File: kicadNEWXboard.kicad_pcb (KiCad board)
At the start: 2 copper layers, 89.7 x 38.1 mm, 24 parts, among them SW1 SW_Push, U1 ATmega32U4-AU, Y1 16MHz

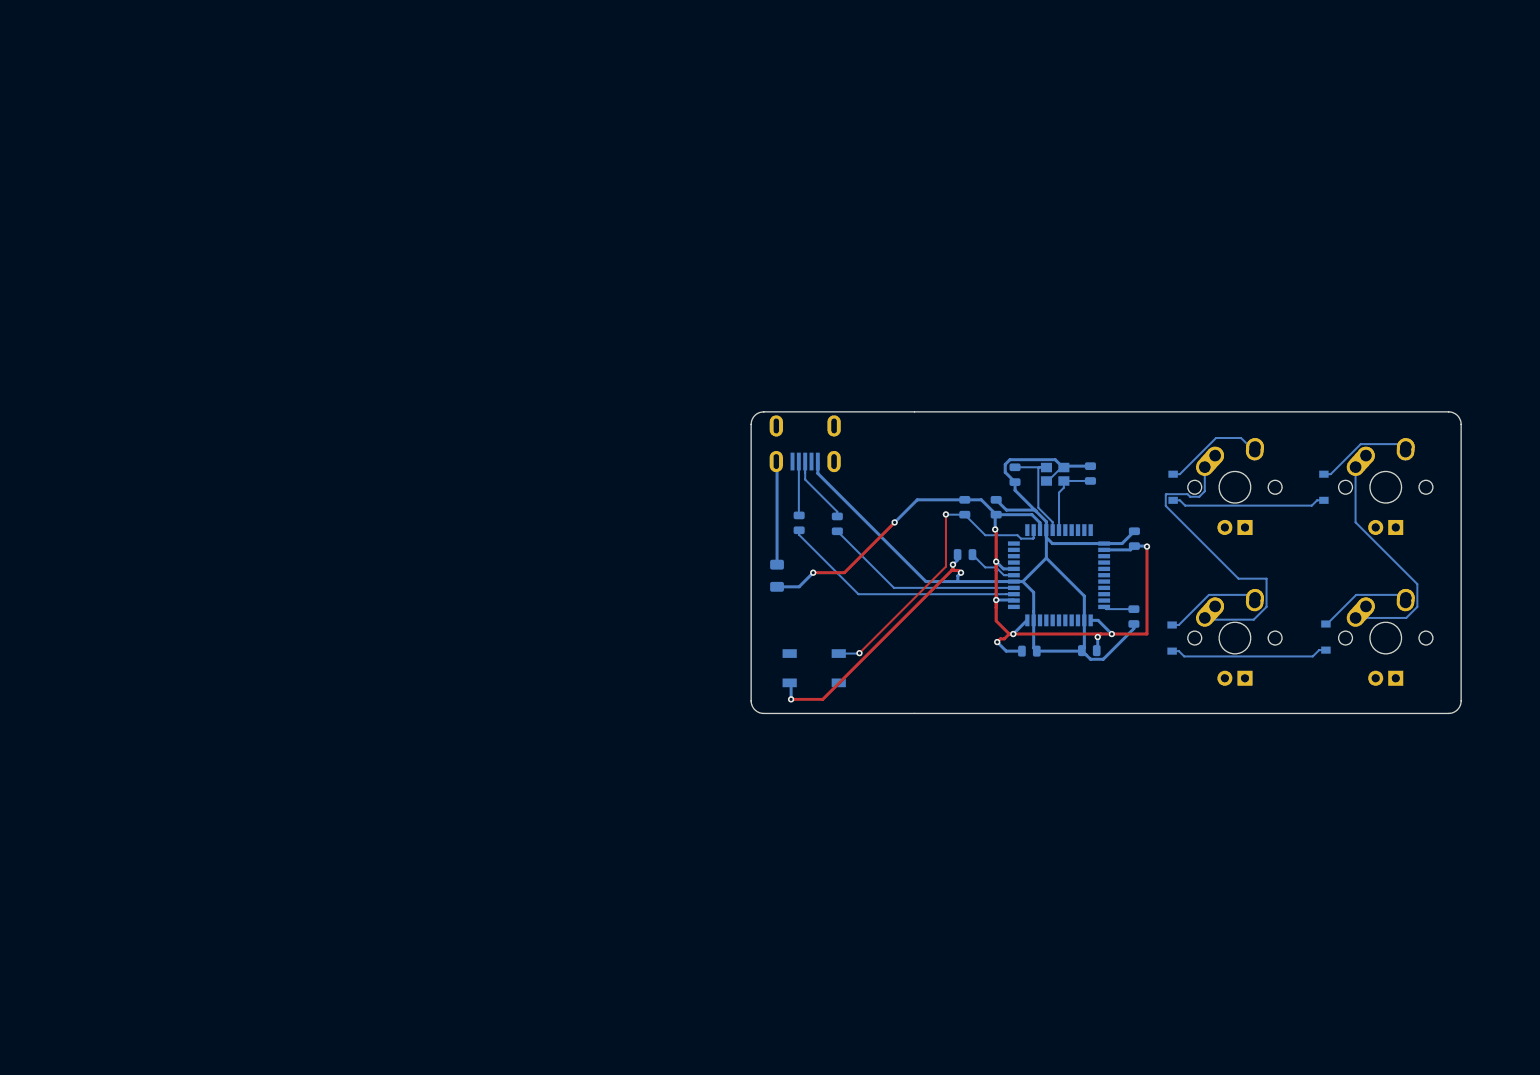
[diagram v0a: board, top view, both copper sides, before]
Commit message: SVG
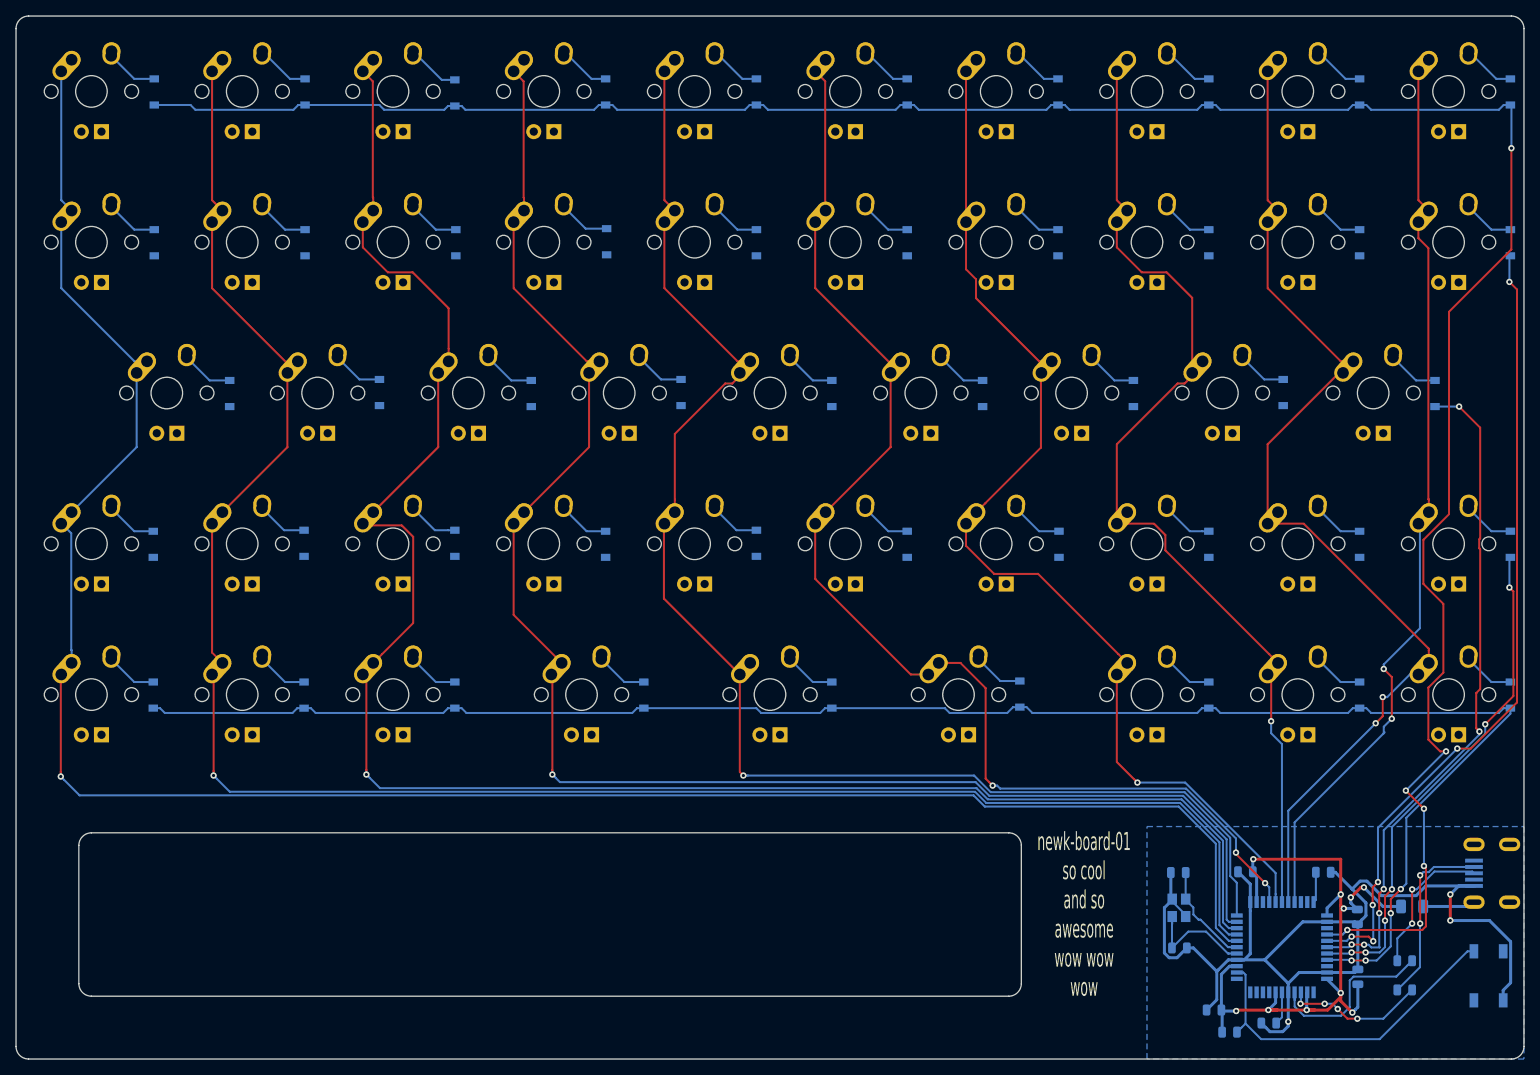
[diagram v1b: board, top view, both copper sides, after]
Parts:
- added D10: SOD-123, Diode_SMD:D_SOD-123, B.Cu at (71.3, 112.0)
- added D11: SOD-123, Diode_SMD:D_SOD-123, B.Cu at (90.4, 35.9)
- added D12: SOD-123, Diode_SMD:D_SOD-123, B.Cu at (90.5, 54.8)
- added D13: SOD-123, Diode_SMD:D_SOD-123, B.Cu at (100.0, 73.9)
- added D14: SOD-123, Diode_SMD:D_SOD-123, B.Cu at (90.4, 92.8)
- added D15: SOD-123, Diode_SMD:D_SOD-123, B.Cu at (90.4, 112.0)
- added D16: SOD-123, Diode_SMD:D_SOD-123, B.Cu at (109.4, 35.8)
- added D17: SOD-123, Diode_SMD:D_SOD-123, B.Cu at (109.5, 54.7)
- added D18: SOD-123, Diode_SMD:D_SOD-123, B.Cu at (118.9, 73.8)
- added D19: SOD-123, Diode_SMD:D_SOD-123, B.Cu at (109.4, 92.9)
- added D20: SOD-123, Diode_SMD:D_SOD-123, B.Cu at (114.2, 112.0)
- added D21: SOD-123, Diode_SMD:D_SOD-123, B.Cu at (128.5, 35.8)
- added D22: SOD-123, Diode_SMD:D_SOD-123, B.Cu at (128.5, 54.8)
- added D23: SOD-123, Diode_SMD:D_SOD-123, B.Cu at (138.0, 73.9)
- added D24: SOD-123, Diode_SMD:D_SOD-123, B.Cu at (128.5, 92.8)
- added D25: SOD-123, Diode_SMD:D_SOD-123, B.Cu at (138.0, 112.0)
- added D26: SOD-123, Diode_SMD:D_SOD-123, B.Cu at (147.5, 35.8)
- added D27: SOD-123, Diode_SMD:D_SOD-123, B.Cu at (147.5, 54.8)
- added D28: SOD-123, Diode_SMD:D_SOD-123, B.Cu at (157.0, 73.9)
- added D29: SOD-123, Diode_SMD:D_SOD-123, B.Cu at (147.5, 92.9)
- added D30: SOD-123, Diode_SMD:D_SOD-123, B.Cu at (161.7, 111.9)
- added D31: SOD-123, Diode_SMD:D_SOD-123, B.Cu at (166.6, 35.8)
- added D32: SOD-123, Diode_SMD:D_SOD-123, B.Cu at (166.6, 54.8)
- added D33: SOD-123, Diode_SMD:D_SOD-123, B.Cu at (176.1, 73.9)
- added D34: SOD-123, Diode_SMD:D_SOD-123, B.Cu at (166.7, 92.9)
- added D35: SOD-123, Diode_SMD:D_SOD-123, B.Cu at (185.6, 112.0)
- added D36: SOD-123, Diode_SMD:D_SOD-123, B.Cu at (185.6, 35.8)
- added D37: SOD-123, Diode_SMD:D_SOD-123, B.Cu at (185.6, 54.8)
- added D38: SOD-123, Diode_SMD:D_SOD-123, B.Cu at (195.0, 73.8)
- added D39: SOD-123, Diode_SMD:D_SOD-123, B.Cu at (185.6, 92.9)
- added D40: SOD-123, Diode_SMD:D_SOD-123, B.Cu at (204.7, 112.0)
- added D41: SOD-123, Diode_SMD:D_SOD-123, B.Cu at (204.7, 35.8)
- added D42: SOD-123, Diode_SMD:D_SOD-123, B.Cu at (204.7, 54.8)
- added D43: SOD-123, Diode_SMD:D_SOD-123, B.Cu at (214.2, 73.9)
- added D44: SOD-123, Diode_SMD:D_SOD-123, B.Cu at (204.7, 92.9)
- added D45: SOD-123, Diode_SMD:D_SOD-123, B.Cu at (223.7, 112.0)
- added D46: SOD-123, Diode_SMD:D_SOD-123, B.Cu at (223.7, 35.8)
- added D47: SOD-123, Diode_SMD:D_SOD-123, B.Cu at (223.7, 54.8)
- added D48: SOD-123, Diode_SMD:D_SOD-123, B.Cu at (223.7, 92.9)
- added D5: SOD-123, Diode_SMD:D_SOD-123, B.Cu at (61.9, 73.9)
- added D6: SOD-123, Diode_SMD:D_SOD-123, B.Cu at (52.3, 92.9)
- added D7: SOD-123, Diode_SMD:D_SOD-123, B.Cu at (52.3, 112.0)
- added D8: SOD-123, Diode_SMD:D_SOD-123, B.Cu at (80.8, 73.8)
- added D9: SOD-123, Diode_SMD:D_SOD-123, B.Cu at (71.3, 92.8)
- added MX10: MX-NoLED, MX_Alps_Hybrid:MX-1U, F.Cu at (63.5, 111.9)
- added MX11: MX-NoLED, MX_Alps_Hybrid:MX-1U, F.Cu at (82.5, 35.7)
- added MX12: MX-NoLED, MX_Alps_Hybrid:MX-1U, F.Cu at (82.5, 54.8)
- added MX13: MX-NoLED, MX_Alps_Hybrid:MX-1U, F.Cu at (92.1, 73.8)
- added MX14: MX-NoLED, MX_Alps_Hybrid:MX-1U, F.Cu at (82.5, 92.9)
- added MX15: MX-NoLED, MX_Alps_Hybrid:MX-1U, F.Cu at (82.5, 111.9)
- added MX16: MX-NoLED, MX_Alps_Hybrid:MX-1U, F.Cu at (101.6, 35.7)
- added MX17: MX-NoLED, MX_Alps_Hybrid:MX-1U, F.Cu at (101.6, 54.8)
- added MX18: MX-NoLED, MX_Alps_Hybrid:MX-1U, F.Cu at (111.1, 73.8)
- added MX19: MX-NoLED, MX_Alps_Hybrid:MX-1U, F.Cu at (101.6, 92.9)
- added MX20: MX-NoLED, MX_Alps_Hybrid:MX-1U, F.Cu at (106.4, 111.9)
- added MX21: MX-NoLED, MX_Alps_Hybrid:MX-1U, F.Cu at (120.7, 35.7)
- added MX22: MX-NoLED, MX_Alps_Hybrid:MX-1U, F.Cu at (120.7, 54.8)
- added MX23: MX-NoLED, MX_Alps_Hybrid:MX-1U, F.Cu at (130.2, 73.8)
- added MX24: MX-NoLED, MX_Alps_Hybrid:MX-1U, F.Cu at (120.7, 92.9)
- added MX25: MX-NoLED, MX_Alps_Hybrid:MX-1U, F.Cu at (130.2, 111.9)
- added MX26: MX-NoLED, MX_Alps_Hybrid:MX-1U, F.Cu at (139.7, 35.7)
- added MX27: MX-NoLED, MX_Alps_Hybrid:MX-1U, F.Cu at (139.7, 54.8)
- added MX28: MX-NoLED, MX_Alps_Hybrid:MX-1U, F.Cu at (149.2, 73.8)
- added MX29: MX-NoLED, MX_Alps_Hybrid:MX-1U, F.Cu at (139.7, 92.9)
- added MX30: MX-NoLED, MX_Alps_Hybrid:MX-1U, F.Cu at (154.0, 111.9)
- added MX31: MX-NoLED, MX_Alps_Hybrid:MX-1U, F.Cu at (158.8, 35.7)
- added MX32: MX-NoLED, MX_Alps_Hybrid:MX-1U, F.Cu at (158.8, 54.8)
- added MX33: MX-NoLED, MX_Alps_Hybrid:MX-1U, F.Cu at (168.3, 73.8)
- added MX34: MX-NoLED, MX_Alps_Hybrid:MX-1U, F.Cu at (158.8, 92.9)
- added MX35: MX-NoLED, MX_Alps_Hybrid:MX-1U, F.Cu at (177.8, 111.9)
- added MX36: MX-NoLED, MX_Alps_Hybrid:MX-1U, F.Cu at (177.8, 35.7)
- added MX37: MX-NoLED, MX_Alps_Hybrid:MX-1U, F.Cu at (177.8, 54.8)
- added MX38: MX-NoLED, MX_Alps_Hybrid:MX-1U, F.Cu at (187.3, 73.8)
- added MX39: MX-NoLED, MX_Alps_Hybrid:MX-1U, F.Cu at (177.8, 92.9)
- added MX40: MX-NoLED, MX_Alps_Hybrid:MX-1U, F.Cu at (196.8, 111.9)
- added MX41: MX-NoLED, MX_Alps_Hybrid:MX-1U, F.Cu at (196.8, 35.7)
- added MX42: MX-NoLED, MX_Alps_Hybrid:MX-1U, F.Cu at (196.8, 54.8)
- added MX43: MX-NoLED, MX_Alps_Hybrid:MX-1U, F.Cu at (206.4, 73.8)
- added MX44: MX-NoLED, MX_Alps_Hybrid:MX-1U, F.Cu at (196.8, 92.9)
- added MX45: MX-NoLED, MX_Alps_Hybrid:MX-1U, F.Cu at (215.9, 111.9)
- added MX46: MX-NoLED, MX_Alps_Hybrid:MX-1U, F.Cu at (215.9, 35.7)
- added MX47: MX-NoLED, MX_Alps_Hybrid:MX-1U, F.Cu at (215.9, 54.8)
- added MX48: MX-NoLED, MX_Alps_Hybrid:MX-1U, F.Cu at (215.9, 92.9)
- added MX5: MX-NoLED, MX_Alps_Hybrid:MX-1U, F.Cu at (54.0, 73.8)
- added MX6: MX-NoLED, MX_Alps_Hybrid:MX-1U, F.Cu at (44.5, 92.9)
- added MX7: MX-NoLED, MX_Alps_Hybrid:MX-1U, F.Cu at (44.5, 111.9)
- added MX8: MX-NoLED, MX_Alps_Hybrid:MX-1U, F.Cu at (73.0, 73.8)
- added MX9: MX-NoLED, MX_Alps_Hybrid:MX-1U, F.Cu at (63.5, 92.9)
- moved MX3 152.9 mm to (63.5, 35.7)
- moved MX4 152.9 mm to (63.5, 54.8)
- moved MX1 152.9 mm to (44.5, 35.7)
- moved MX2 152.9 mm to (44.5, 54.8)
- moved D4 138.3 mm to (71.4, 54.8)
- moved D1 138.1 mm to (52.4, 35.8)
- moved D3 138.1 mm to (71.4, 35.8)
- moved D2 137.9 mm to (52.4, 54.8)
- moved USB1 105.4 mm to (223.6, 134.5), turned to 180 degrees
- moved R1 96.6 mm to (210.4, 149.2), turned to 180 degrees
- moved SW1 93.6 mm to (220.9, 147.4), turned to 270 degrees
- moved R2 90.5 mm to (210.4, 145.5), turned to 180 degrees
- moved F1 90.5 mm to (211.3, 138.7), turned to 0 degrees
- moved R3 74.3 mm to (188.2, 154.6), turned to 180 degrees
- moved C6 70.5 mm to (193.2, 153.4)
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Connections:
- U1 pad 18: Net-(U1-Pad18) -> COL0
- U1 pad 19: Net-(U1-Pad19) -> COL1
- U1 pad 20: Net-(U1-Pad20) -> COL2
- U1 pad 21: Net-(U1-Pad21) -> COL3
- U1 pad 22: Net-(U1-Pad22) -> COL4
- U1 pad 26: Net-(U1-Pad26) -> COL5
- U1 pad 27: Net-(U1-Pad27) -> COL6
- U1 pad 28: Net-(U1-Pad28) -> COL7
- U1 pad 29: Net-(U1-Pad29) -> COL8
- U1 pad 30: Net-(U1-Pad30) -> COL9
- U1 pad 37: Net-(U1-Pad37) -> ROW0
- U1 pad 38: Net-(U1-Pad38) -> ROW1
- U1 pad 39: Net-(U1-Pad39) -> ROW2
- U1 pad 40: Net-(U1-Pad40) -> ROW3
- U1 pad 41: Net-(U1-Pad41) -> ROW4
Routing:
- net ROW0: track 19.6 -> 303.5 mm, vias 0 -> 6
- net COL2: track 0.00 -> 227.0 mm, vias 0 -> 1
- net ROW4: track 0.00 -> 220.8 mm, vias 0 -> 4
- net COL0: track 38.5 -> 256.6 mm, vias 0 -> 1
- net COL1: track 29.3 -> 236.8 mm, vias 0 -> 1
- net COL3: track 0.00 -> 195.1 mm, vias 0 -> 1
- net COL4: track 0.00 -> 173.6 mm, vias 0 -> 1
- net COL5: track 0.00 -> 155.6 mm, vias 0 -> 3
- net COL6: track 0.00 -> 132.9 mm, vias 0 -> 1
- net COL8: track 0.00 -> 129.7 mm, vias 0 -> 2
- net COL7: track 0.00 -> 125.4 mm, vias 0 -> 1
- net COL9: track 0.00 -> 110.8 mm, vias 0 -> 2
- net ROW2: track 0.00 -> 85.1 mm, vias 0 -> 6
- net ROW1: track 20.0 -> 101.9 mm, vias 0 -> 6
- net ROW3: track 0.00 -> 63.9 mm, vias 0 -> 6
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- added copper zone on B.Cu, net GND
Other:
- board size 89.7 x 38.1 mm -> 190.5 x 131.8 mm
- board text added: "newk-board-01 so cool and so awesome wow wow wow"
